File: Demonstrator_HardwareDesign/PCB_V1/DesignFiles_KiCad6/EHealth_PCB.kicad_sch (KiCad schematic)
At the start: 24 parts, among them J1-AnalogSensors1 Conn_01x05, J3-MagneticInterconnect1 Conn_01x08, J4-OffTheShelf-Digital1 Conn_02x06_Counter_Clockwise, J5-Power1 Conn_01x03

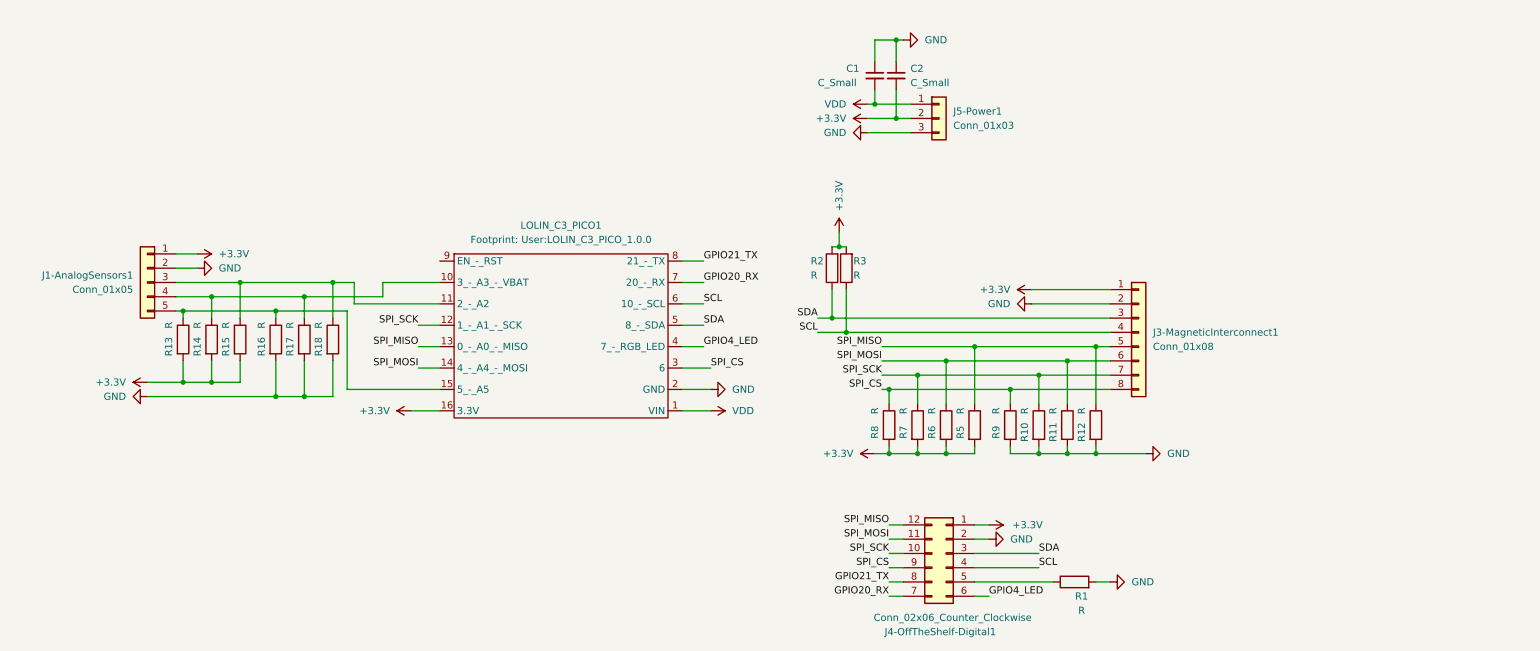
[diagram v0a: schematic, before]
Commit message: aangepaste pcb layout
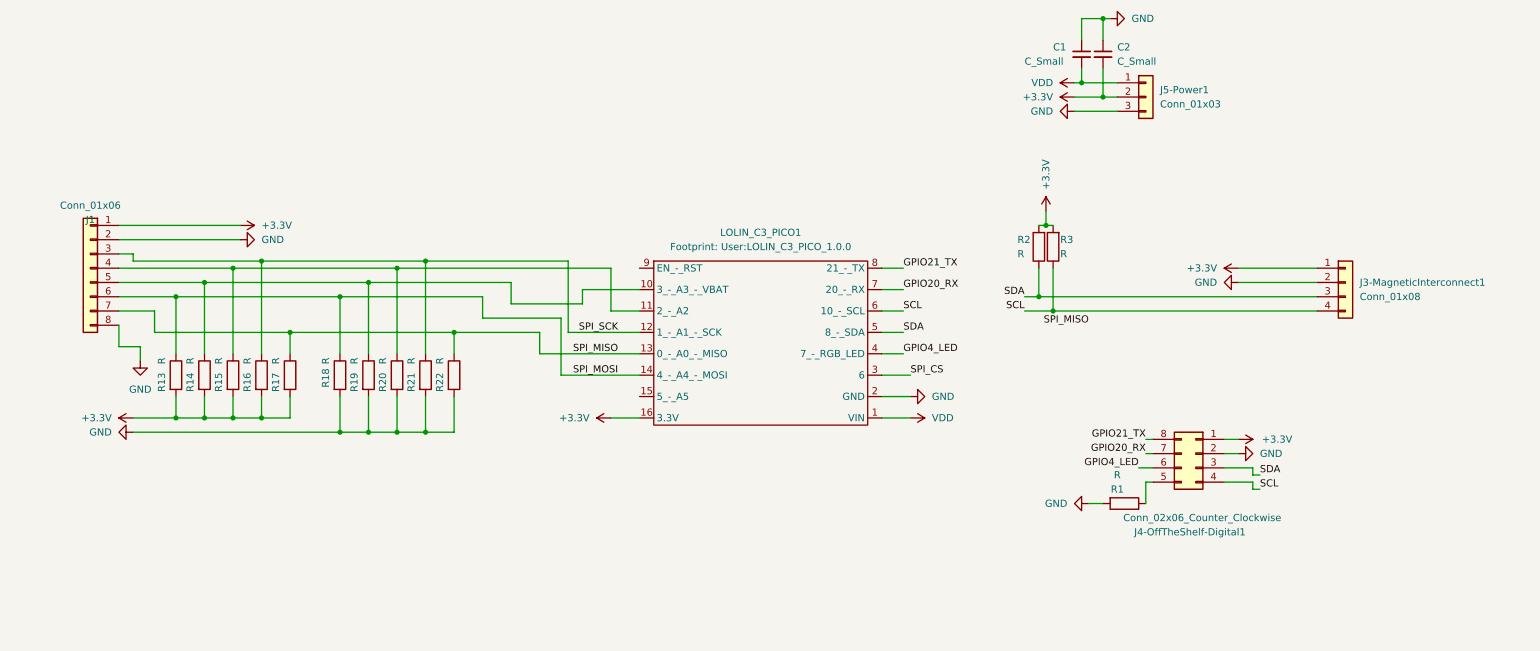
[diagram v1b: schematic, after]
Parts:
- removed J1-AnalogSensors1: Conn_01x05, Connector_PinHeader_2.54mm:PinHeader_1x05_P2.54mm_Vertical, symbol Connector_Generic:Conn_01x05
- removed R10, R11, R12, R5, R6, R7, R8, R9: R, Resistor_SMD:R_0805_2012Metric_Pad1.20x1.40mm_HandSolder, symbol Device:R
- added J1: Conn_01x06, Connector_PinHeader_2.54mm:PinHeader_2x04_P2.54mm_Vertical, symbol Connector_Generic:Conn_01x08
- added R16, R17, R21, R22: R, Resistor_SMD:R_0805_2012Metric_Pad1.20x1.40mm_HandSolder, symbol Device:R
- J3-MagneticInterconnect1: footprint Connector_JST:JST_VH_B8P-VH-B_1x08_P3.96mm_Vertical -> Connector_JST:JST_VH_B4P-VH-B_1x04_P3.96mm_Vertical; symbol Connector_Generic:Conn_01x08 -> Connector_Generic:Conn_01x04
- J4-OffTheShelf-Digital1: footprint Connector_PinSocket_2.54mm:PinSocket_2x06_P2.54mm_Vertical -> Connector_PinSocket_2.54mm:PinSocket_2x04_P2.54mm_Vertical; symbol Connector_Generic:Conn_02x06_Counter_Clockwise -> Connector_Generic:Conn_02x04_Counter_Clockwise
- renumbered R16 to R18, R17 to R19, R18 to R20
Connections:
- net +3.3V: now also J1.1 (Pin_1), R16.2, R17.2
- net GND: now also J1.2 (Pin_2), J1.8 (Pin_8), R21.2, R22.2
- net SPI_CS: no longer J3-MagneticInterconnect1.8 (Pin_8), J4-OffTheShelf-Digital1.9 (Pin_9)
- net SPI_MISO: now also J1.7 (Pin_7), R17.1, R22.1; no longer J3-MagneticInterconnect1.5 (Pin_5), J4-OffTheShelf-Digital1.12 (Pin_12)
- net SPI_MOSI: now also R13.1, R18.1, J1.6 (Pin_6); no longer J3-MagneticInterconnect1.6 (Pin_6), J4-OffTheShelf-Digital1.11 (Pin_11)
- net SPI_SCK: now also J1.3 (Pin_3), R16.1, R21.1; no longer J3-MagneticInterconnect1.7 (Pin_7), J4-OffTheShelf-Digital1.10 (Pin_10)
- net at LOLIN_C3_PICO1.10 (3_-_A3_-_VBAT), R14.1, R19.1: now also J1.5 (Pin_5)
- net at LOLIN_C3_PICO1.11 (2_-_A2), R15.1, R20.1: now also J1.4 (Pin_4)
- now unconnected: LOLIN_C3_PICO1.15 (5_-_A5)
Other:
- moved on the sheet: C1, C2, J5-Power1, LOLIN_C3_PICO1, R1, R13, R14, R15, R18, R19, R2, R20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
